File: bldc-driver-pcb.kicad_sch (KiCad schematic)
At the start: 0 parts

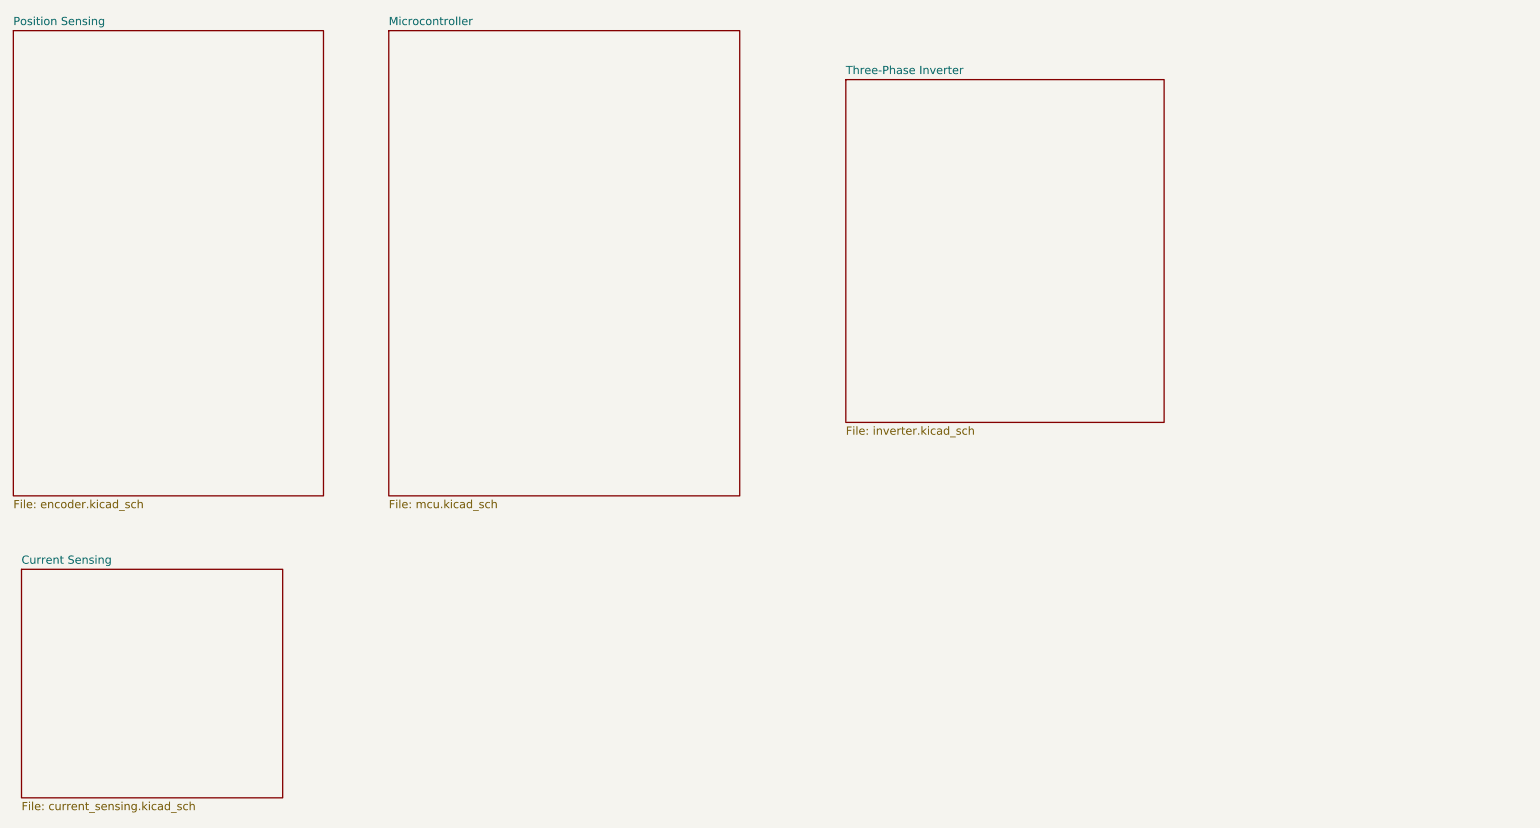
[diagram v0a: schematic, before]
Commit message: Initial routing
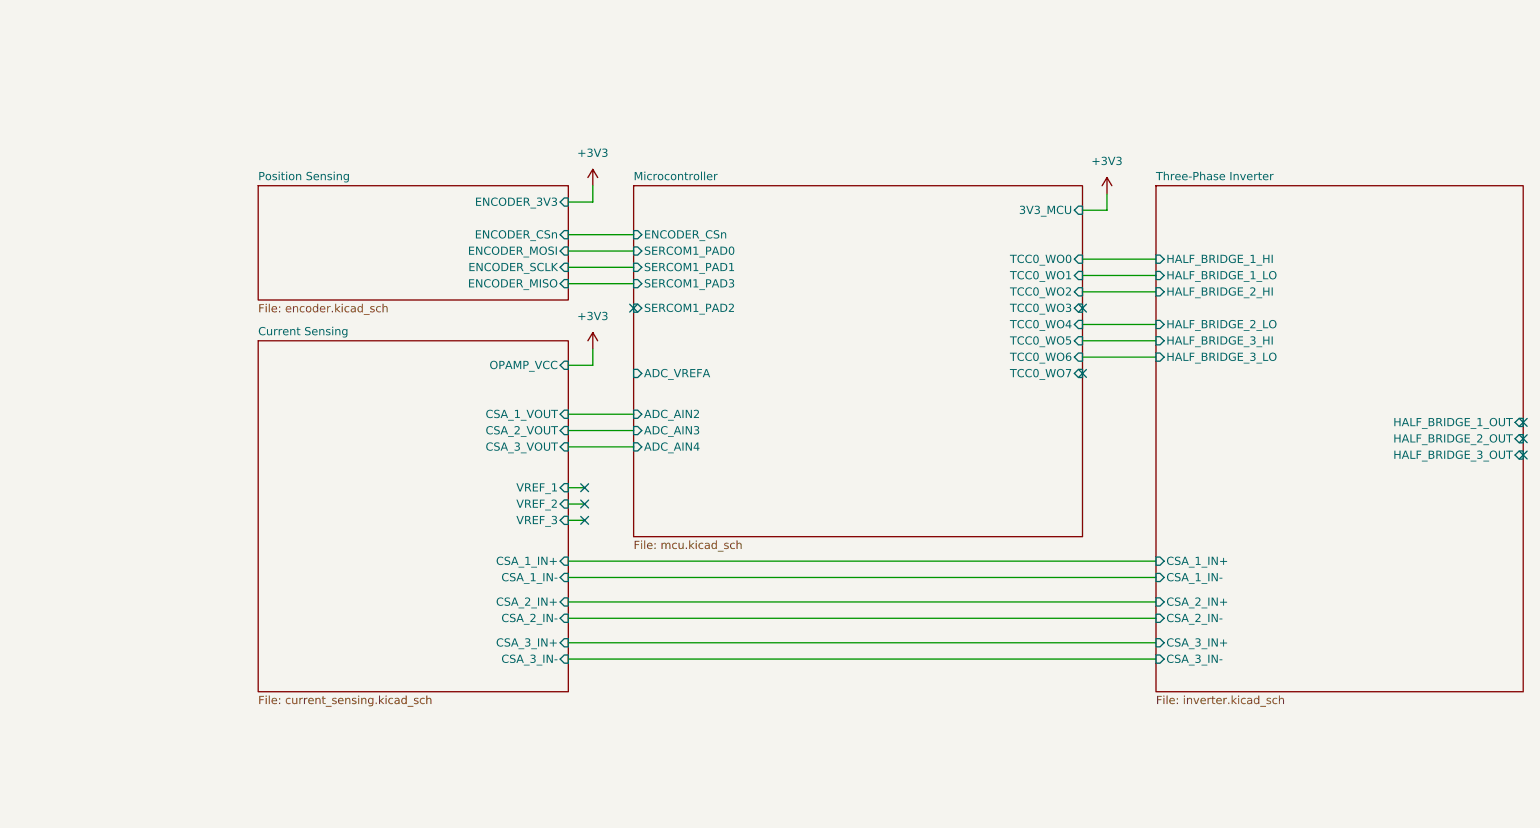
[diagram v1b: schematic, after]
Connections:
- no-connect marks 0 -> 9
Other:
- sheet Current Sensing ports: added CSA_1_IN+, CSA_1_IN-, CSA_1_VOUT, CSA_2_IN+, CSA_2_IN-, CSA_2_VOUT, CSA_3_IN+, CSA_3_IN-, CSA_3_VOUT, OPAMP_VCC, VREF_1, VREF_2, VREF_3; removed none
- sheet Microcontroller ports: added 3V3_MCU, ADC_AIN2, ADC_AIN3, ADC_AIN4, ADC_VREFA, ENCODER_CSn, SERCOM1_PAD0, SERCOM1_PAD1, SERCOM1_PAD2, SERCOM1_PAD3, TCC0_WO0, TCC0_WO1, TCC0_WO2, TCC0_WO3, TCC0_WO4, TCC0_WO5, TCC0_WO6, TCC0_WO7; removed none
- sheet Position Sensing ports: added ENCODER_3V3, ENCODER_CSn, ENCODER_MISO, ENCODER_MOSI, ENCODER_SCLK; removed none
- sheet Three-Phase Inverter ports: added CSA_1_IN+, CSA_1_IN-, CSA_2_IN+, CSA_2_IN-, CSA_3_IN+, CSA_3_IN-, HALF_BRIDGE_1_HI, HALF_BRIDGE_1_LO, HALF_BRIDGE_1_OUT, HALF_BRIDGE_2_HI, HALF_BRIDGE_2_LO, HALF_BRIDGE_2_OUT, HALF_BRIDGE_3_HI, HALF_BRIDGE_3_LO, HALF_BRIDGE_3_OUT; removed none
